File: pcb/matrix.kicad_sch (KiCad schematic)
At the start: 69 parts, among them J1 Conn_01x02, J2 USB_C_Receptacle_USB2.0_14P, SW1 SW_Push, SW2 SW_Push, SW3 SW_Push, SW4 SW_Push, U1 ESP32-S3-MINI-1U, U2 XC6206PxxxMR

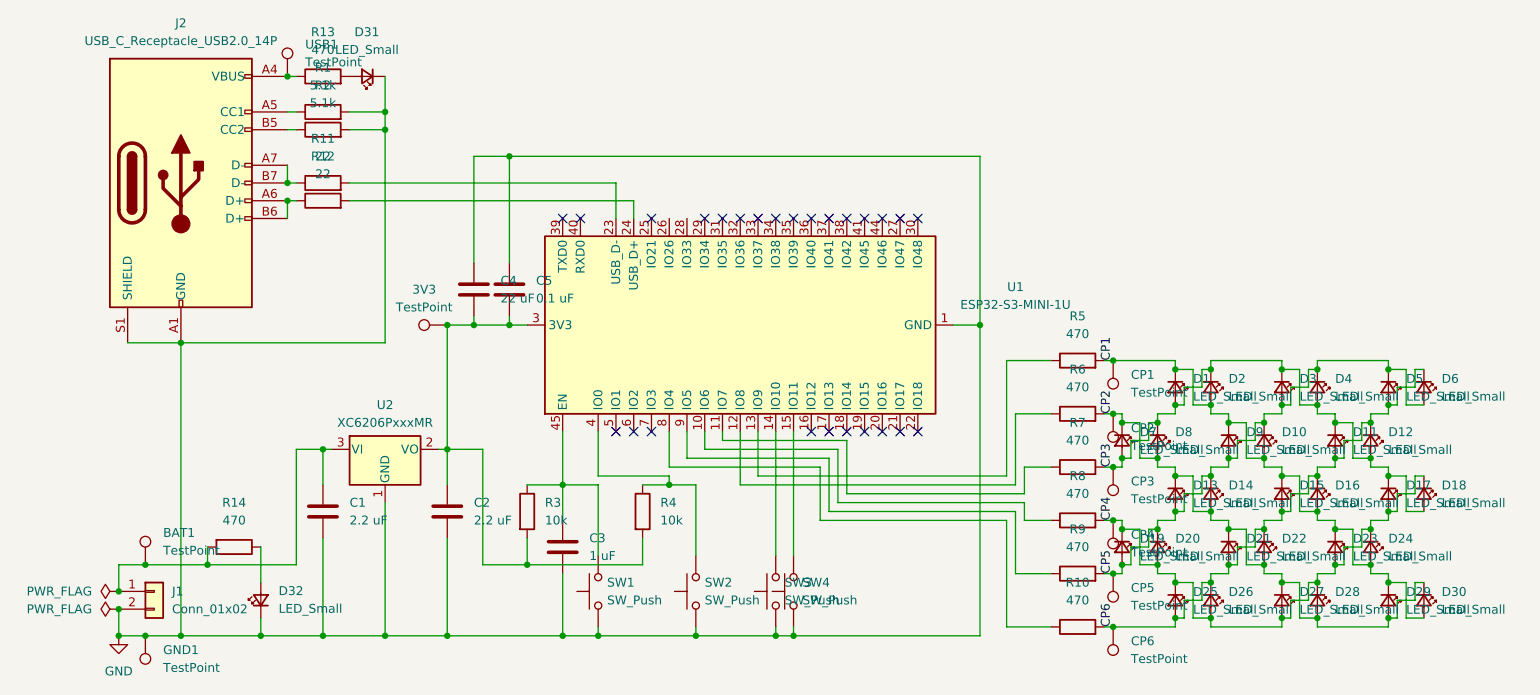
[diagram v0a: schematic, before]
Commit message: Replace components
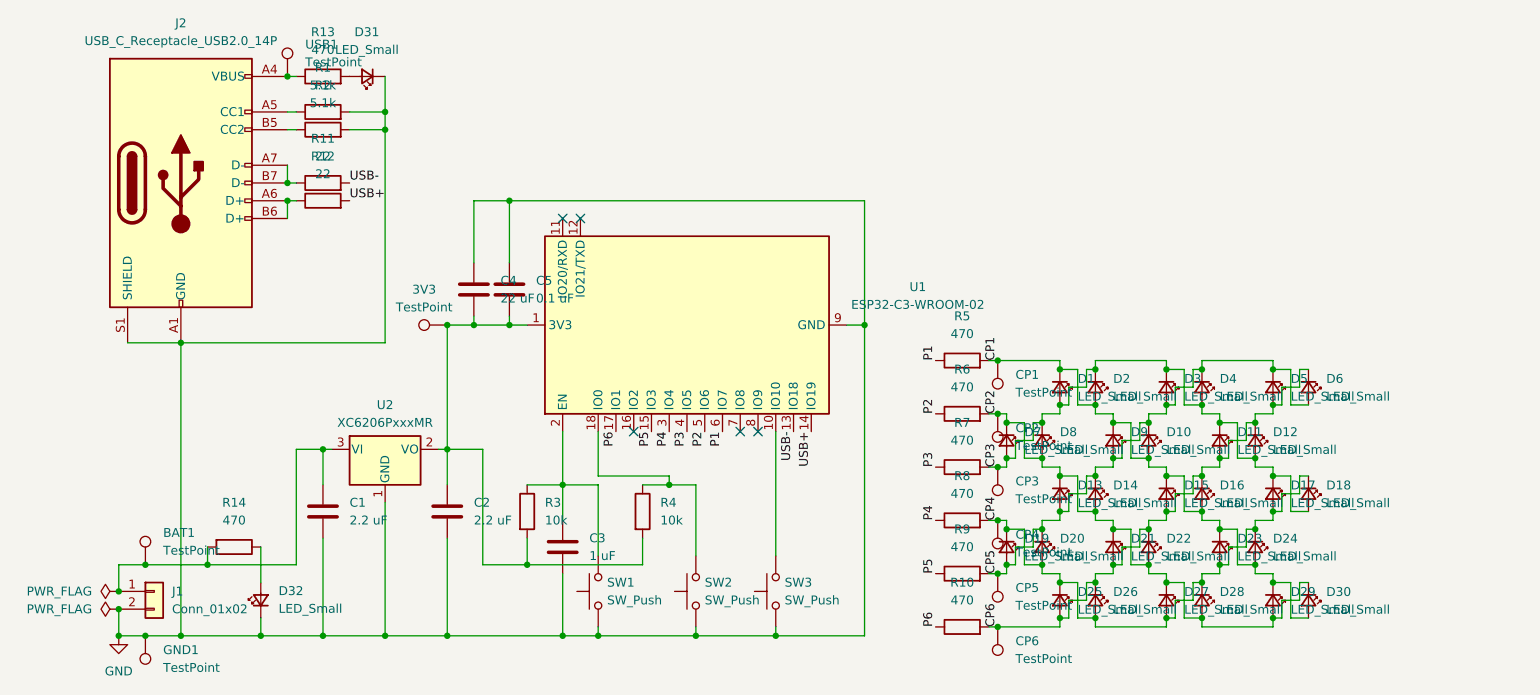
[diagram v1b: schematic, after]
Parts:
- removed SW4: SW_Push, Button_Switch_SMD:SW_SPST_PTS810, symbol Switch:SW_Push
- removed U1: ESP32-S3-MINI-1U, RF_Module:ESP32-S2-MINI-1U, symbol RF_Module:ESP32-S3-MINI-1U
- added U1: ESP32-C3-WROOM-02, RF_Module:ESP32-C3-WROOM-02, symbol RF_Module:ESP32-C3-WROOM-02
- SW1, SW2, SW3: footprint Button_Switch_SMD:SW_SPST_PTS810 -> Button_Switch_SMD:SW_SPST_TS-1088-xR020
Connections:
- net GND: now also U1.19 (GND), U1.9 (GND)
- net at 3V3.1, C2.1, C4.2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: now also U1.1 (3V3)
- net P5: now reaches R9.1
- net P5: now also U1.15 (IO3)
- net P4: now reaches R8.1
- net P4: now also U1.3 (IO4)
- net P3: now reaches R7.1
- net P3: now also U1.4 (IO5)
- net P2: now reaches R6.1
- net P2: now also U1.5 (IO6)
- net P1: now reaches R5.1
- net P1: now also U1.6 (IO7)
- net at SW3.2: now also U1.10 (IO10)
- net USB-: now reaches R11.2
- net USB-: now also U1.13 (IO18)
- net USB+: now reaches R12.2
- net USB+: now also U1.14 (IO19)
- net at R4.1, SW2.2: now also U1.18 (IO0)
- net at C3.1, R3.1, SW1.2: now also U1.2 (EN)
- net P6: now reaches R10.1
- net P6: now also U1.17 (IO1)
- no-connect marks 26 -> 5
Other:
- moved on the sheet: CP1, CP2, CP3, CP4, CP5, CP6, D1, D10, D11, D12, D13, D14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
